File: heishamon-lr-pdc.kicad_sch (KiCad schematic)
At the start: 30 parts, among them CN1 S05B-XASK-1(LF)(SN), CN2 S05B-XASK-1(LF)(SN), J1 Conn_01x04_Pin, J2 ESP_SER_DBG, J3 VCC_IN, U1 ISO7762FDW, U2 B1205S-2WR2_C2992386, U3 ESP32-C3-DevKitC-02

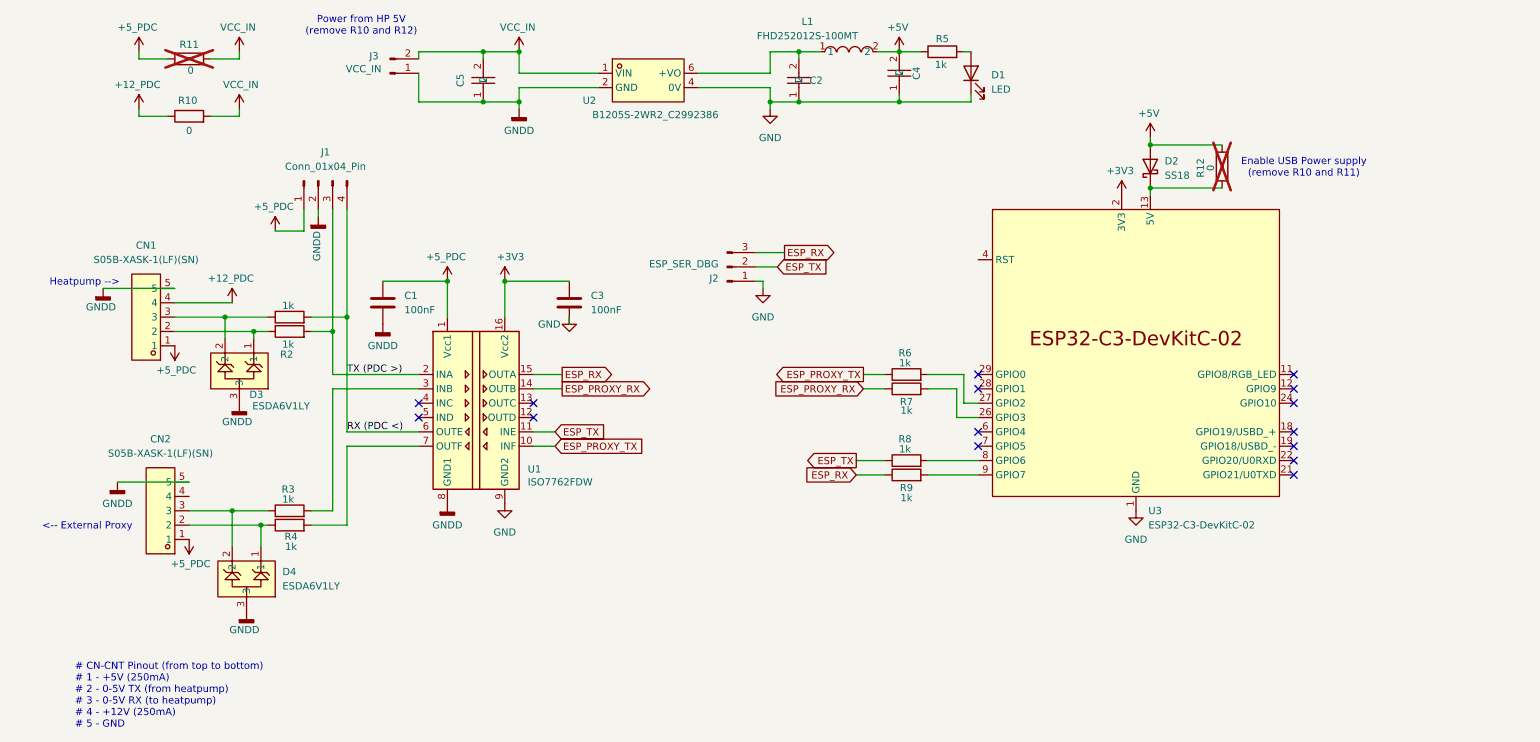
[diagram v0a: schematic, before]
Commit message: Update
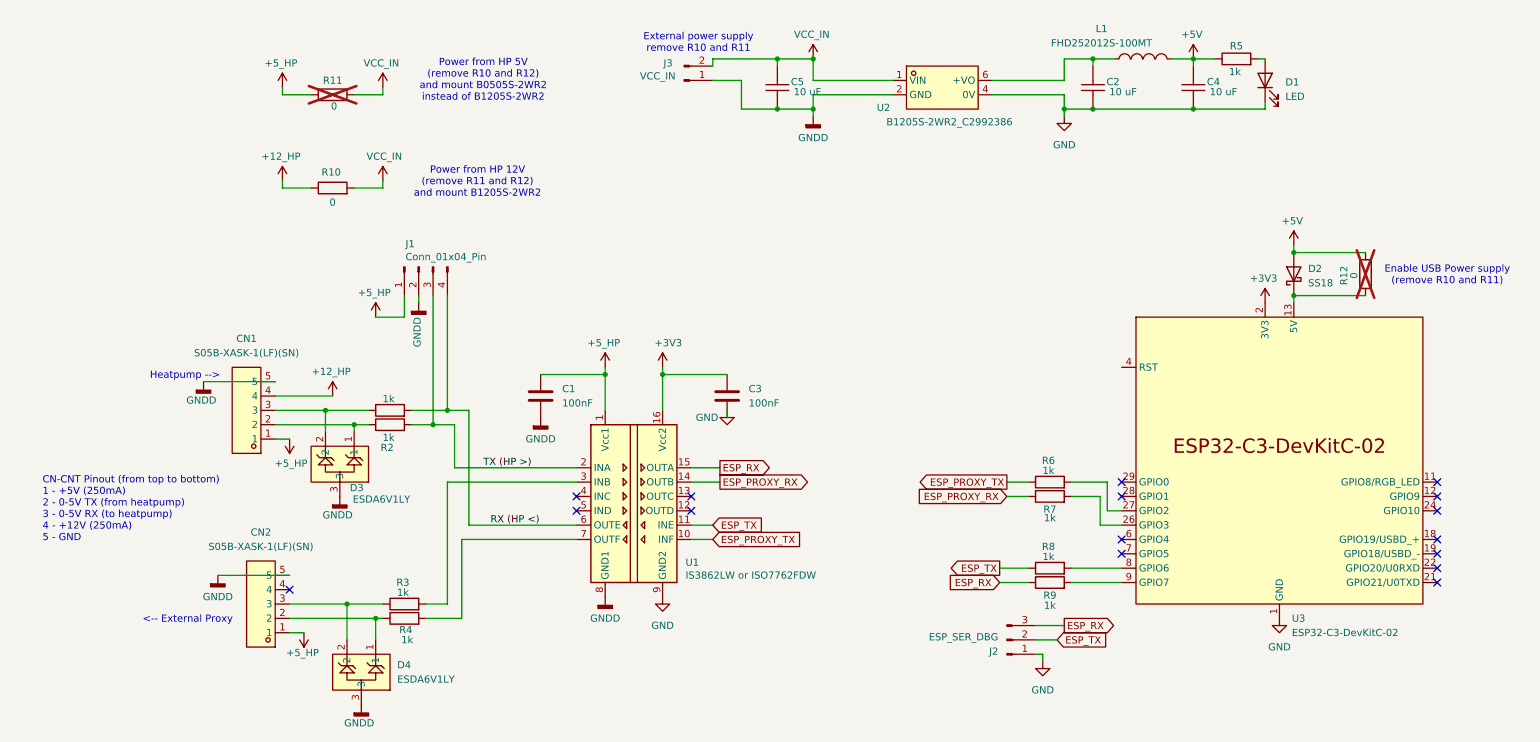
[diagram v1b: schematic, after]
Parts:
- C2, C4, C5: value CL21A475KAQNNNE -> 10 uF; LCSC Part C1779 -> C15850
- U1: value ISO7762FDW -> IS3862LW or ISO7762FDW; LCSC (none) -> C20598881
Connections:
- net +12_PDC renamed +12_HP
- net +5_PDC renamed +5_HP
- net RX (PDC <) renamed RX (HP <)
- net RX (HP <): no longer J1.3 (Pin_3), R2.2, U1.2 (INA)
- new net TX (HP >): J1.3 (Pin_3), R2.2, U1.2 (INA)
- no-connect marks 15 -> 16
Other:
- note added: "CN-CNT Pinout (from top to bottom) 1 - +5V (250mA) 2 - 0-5V TX (from heatpump) 3 - 0-5V RX (to heatpump) 4 - +12V (250mA) 5 - GND"
- note added: "External power supply remove R10 and R11"
- note added: "Power from HP 12V (remove R11 and R12) and mount B1205S-2WR2"
- note added: "Power from HP 5V (remove R10 and R12) and mount B0505S-2WR2 instead of B1205S-2WR2"
- note removed: "# CN-CNT Pinout (from top to bottom) # 1 - +5V (250mA) # 2 - 0-5V TX (from heatpump) # 3 - 0-5V RX (to heatpump) # 4 - +12V (250mA) # 5 - GND"
- note removed: "Power from HP 5V (remove R10 and R12)"
- moved on the sheet: C1, C3, CN1, CN2, D1, D2, D3, D4, J1, J2, J3, R10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
